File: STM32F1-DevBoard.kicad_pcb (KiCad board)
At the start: 2 copper layers, 20.3 x 50.8 mm, 39 parts, among them J1 USB_C_Receptacle_USB2.0, SW1 SW_Push, SW2 SW_Push, U1 STM32F103C8T6, U2 AMS1117-3.3, U3 W25Q32JVSS

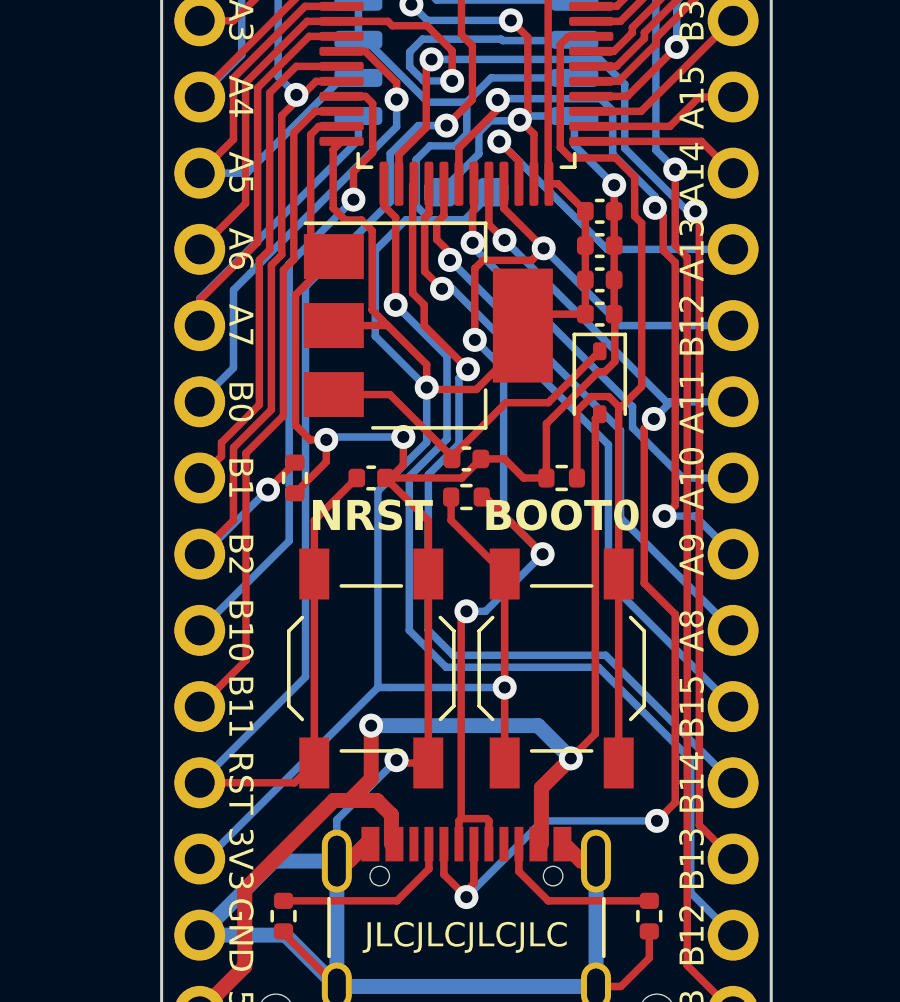
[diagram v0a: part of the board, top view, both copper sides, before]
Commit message: Add files via upload
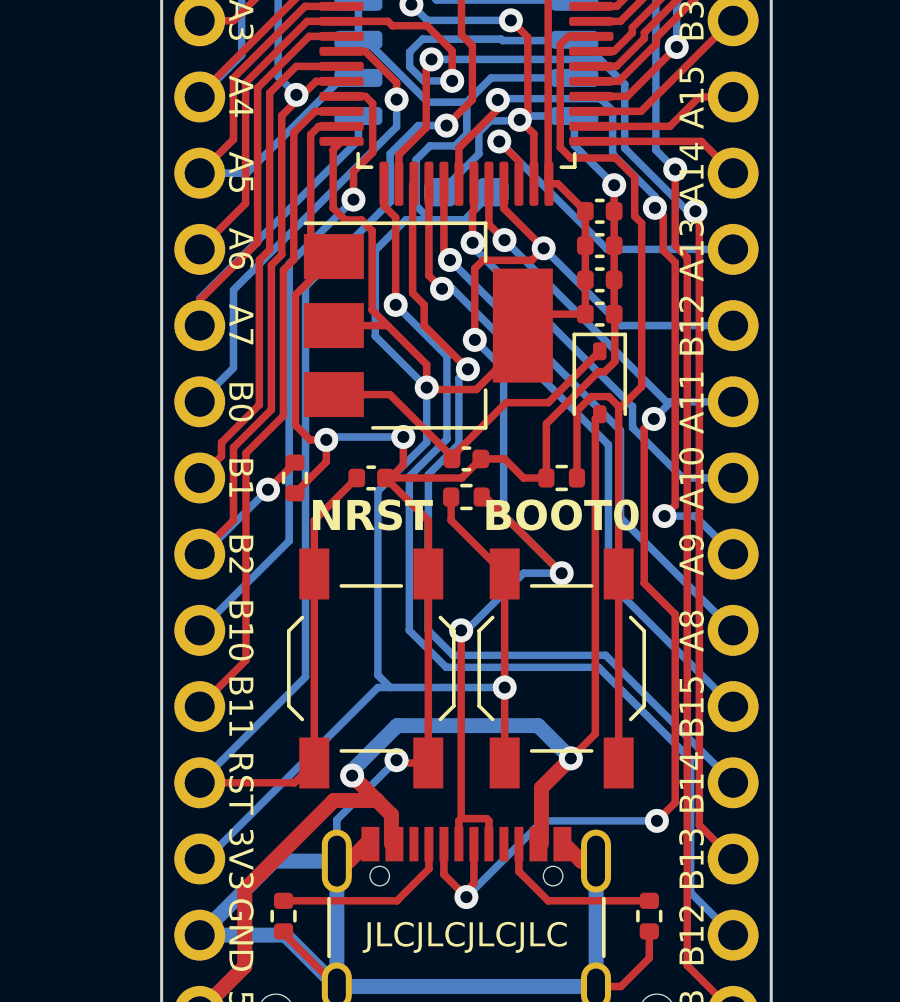
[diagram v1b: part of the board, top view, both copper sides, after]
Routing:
- net PA12: track 38.9 -> 40.8 mm
